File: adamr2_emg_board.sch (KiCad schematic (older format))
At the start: 5 parts, among them J1 Screw_Terminal_01x02, J2 Conn_01x02, J3 Screw_Terminal_01x02, K1 G6C-1114P-US

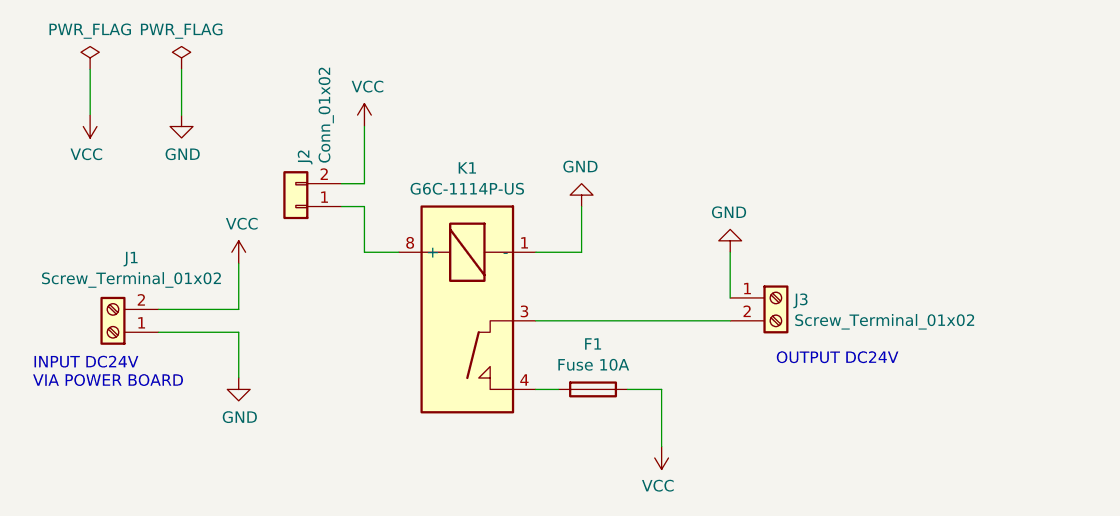
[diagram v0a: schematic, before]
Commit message: Update
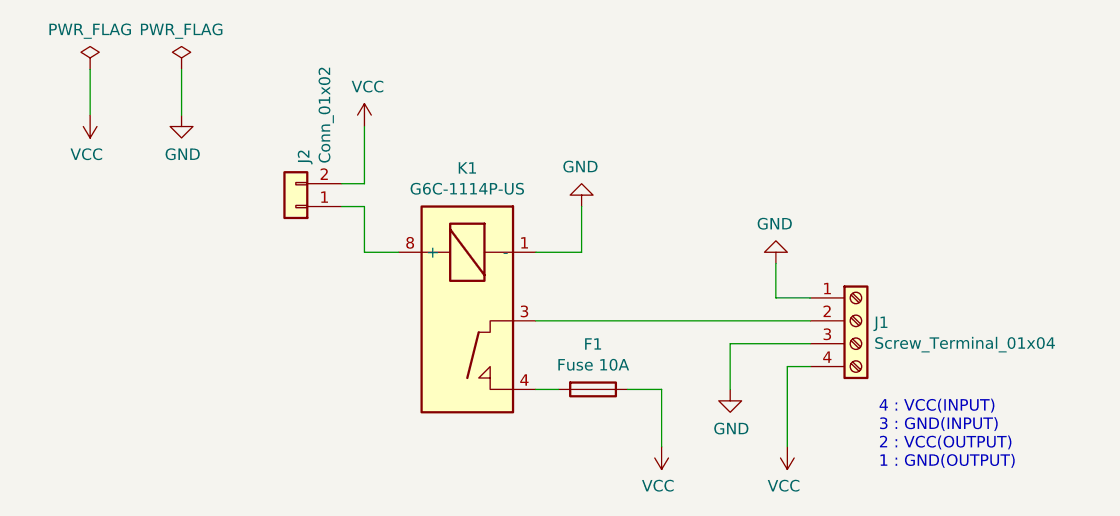
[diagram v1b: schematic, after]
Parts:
- removed J1, J3: Screw_Terminal_01x02, adamr2_footprints:OSTYK21102030, symbol Connector:Screw_Terminal_01x02
- added J1: Screw_Terminal_01x04, adamr2_footprints:OSTYK21104030, symbol Connector:Screw_Terminal_01x04
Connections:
- net GND: now also J1.1 (Pin_1), J1.3 (Pin_3)
- net VCC: now also J1.4 (Pin_4)
- net at K1.3: now also J1.2 (Pin_2)
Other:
- note added: "4 : VCC(INPUT)\n3 : GND(INPUT)\n2 : VCC(OUTPUT)\n1 : GND(OUTPUT)"
- note removed: "INPUT DC24V\nVIA POWER BOARD"
- note removed: "OUTPUT DC24V"
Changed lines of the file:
@@
 L power:GND #PWR02
 U 1 1 5F249FAF
-P 5100 3600
-F 0 "#PWR02" H 5100 3350 50  0001 C CNN
-F 1 "GND" H 5105 3427 50  0000 C CNN
-F 2 "" H 5100 3600 50  0001 C CNN
-F 3 "" H 5100 3600 50  0001 C CNN
-	1    5100 3600
+P 7250 3650
+F 0 "#PWR02" H 7250 3400 50  0001 C CNN
+F 1 "GND" H 7255 3477 50  0000 C CNN
+F 2 "" H 7250 3650 50  0001 C CNN
+F 3 "" H 7250 3650 50  0001 C CNN
+	1    7250 3650
 	1    0    0    -1
 $EndComp
-$Comp
-L Connector:Screw_Terminal_01x02 J1
-U 1 1 5F24A5AD
-P 4550 3400
-F 0 "J1" H 4468 3075 50  0000 C CNN
-F 1 "Screw_Terminal_01x02" H 4468 3166 50  0000 C CNN
-F 2 "adamr2_footprints:OSTYK21102030" H 4550 3400 50  0001 C CNN
-F 3 "~" H 4550 3400 50  0001 C CNN
-	1    4550 3400
-	-1   0    0    1
-$EndComp
-Text Notes 4200 3650 0    50   ~ 0
-INPUT DC24V\nVIA POWER BOARD
 $Comp
 L power:VCC #PWR03
@@
 	-1   0    0    1
 $EndComp
-Text Notes 7450 3550 0    50   ~ 0
-OUTPUT DC24V
 $Comp
 L power:VCC #PWR0102
 U 1 1 5F266BB5
-P 5100 3100
-F 0 "#PWR0102" H 5100 2950 50  0001 C CNN
-F 1 "VCC" H 5115 3273 50  0000 C CNN
-F 2 "" H 5100 3100 50  0001 C CNN
-F 3 "" H 5100 3100 50  0001 C CNN
-	1    5100 3100
-	1    0    0    -1
+P 7500 3900
+F 0 "#PWR0102" H 7500 3750 50  0001 C CNN
+F 1 "VCC" H 7515 4073 50  0000 C CNN
+F 2 "" H 7500 3900 50  0001 C CNN
+F 3 "" H 7500 3900 50  0001 C CNN
+	1    7500 3900
+	-1   0    0    1
 $EndComp
 $Comp
@@
 	4850 2250 4850 2450
 $Comp
-L adamr2_symbols:G6C-1114P-US K1
-U 1 1 5F23BF02
-P 6100 3250
-F 0 "K1" V 5533 3250 50  0000 C CNN
-F 1 "G6C-1114P-US" V 5624 3250 50  0000 C CNN
-F 2 "adamr2_footprints:G6C-1114P-US" H 6450 3200 50  0001 L CNN
-F 3 "https://omronfs.omron.com/ja_JP/ecb/products/pdf/g6c.pdf" H 6100 3250 50  0001 C CNN
-	1    6100 3250
-	0    1    1    0
-$EndComp
-$Comp
 L Connector_Generic:Conn_01x02 J2
 U 1 1 5F24B365
@@
 	5650 2750 5650 2500
 Wire Wire Line
-	4750 3300 5100 3300
-Wire Wire Line
-	5100 3300 5100 3100
-Wire Wire Line
-	5100 3400 5100 3600
-Wire Wire Line
-	4750 3400 5100 3400
-Wire Wire Line
 	6500 3650 6400 3650
-Wire Wire Line
-	7250 3350 6400 3350
 $Comp
 L power:GND #PWR05
 U 1 1 5F254AEA
-P 7250 3050
-F 0 "#PWR05" H 7250 2800 50  0001 C CNN
-F 1 "GND" H 7255 2877 50  0000 C CNN
-F 2 "" H 7250 3050 50  0001 C CNN
-F 3 "" H 7250 3050 50  0001 C CNN
-	1    7250 3050
+P 7450 3100
+F 0 "#PWR05" H 7450 2850 50  0001 C CNN
+F 1 "GND" H 7455 2927 50  0000 C CNN
+F 2 "" H 7450 3100 50  0001 C CNN
+F 3 "" H 7450 3100 50  0001 C CNN
+	1    7450 3100
 	-1   0    0    1
 $EndComp
-$Comp
-L Connector:Screw_Terminal_01x02 J3
-U 1 1 5F24ACF4
-P 7450 3250
-F 0 "J3" H 7530 3242 50  0000 L CNN
-F 1 "Screw_Terminal_01x02" H 7530 3151 50  0000 L CNN
-F 2 "adamr2_footprints:OSTYK21102030" H 7450 3250 50  0001 C CNN
-F 3 "~" H 7450 3250 50  0001 C CNN
-	1    7450 3250
-	1    0    0    -1
-$EndComp
-Wire Wire Line
-	7250 3050 7250 3250
 Wire Wire Line
 	6800 3650 6950 3650
 Wire Wire Line
 	6950 3650 6950 3900
+$Comp
+L Connector:Screw_Terminal_01x04 J1
+U 1 1 5F2A9452
+P 7800 3350
+F 0 "J1" H 7880 3342 50  0000 L CNN
+F 1 "Screw_Terminal_01x04" H 7880 3251 50  0000 L CNN
+F 2 "adamr2_footprints:OSTYK21104030" H 7800 3350 50  0001 C CNN
+F 3 "~" H 7800 3350 50  0001 C CNN
+	1    7800 3350
+	1    0    0    -1
+$EndComp
+Text Notes 7900 4000 0    50   ~ 0
+4 : VCC(INPUT)\n3 : GND(INPUT)\n2 : VCC(OUTPUT)\n1 : GND(OUTPUT)
+Wire Wire Line
+	6400 3350 7600 3350
+Wire Wire Line
+	7450 3100 7450 3250
+Wire Wire Line
+	7450 3250 7600 3250
+Wire Wire Line
+	7600 3550 7500 3550
+Wire Wire Line
+	7500 3550 7500 3900
+Wire Wire Line
+	7600 3450 7250 3450
+Wire Wire Line
+	7250 3450 7250 3650
+$Comp
+L adamr2_symbols:G6C-1114P-US K1
+U 1 1 5F23BF02
+P 6100 3250
+F 0 "K1" V 5533 3250 50  0000 C CNN
+F 1 "G6C-1114P-US" V 5624 3250 50  0000 C CNN
+F 2 "adamr2_footprints:G6C-1114P-US" H 6450 3200 50  0001 L CNN
+F 3 "https://omronfs.omron.com/ja_JP/ecb/products/pdf/g6c.pdf" H 6100 3250 50  0001 C CNN
+	1    6100 3250
+	0    1    1    0
+$EndComp
 $EndSCHEMATC

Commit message: Update: ヒューズホルダの種類を変更した
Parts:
- F1: footprint adamr2_footprints:FUC-03A -> adamr2_footprints:F-60-A
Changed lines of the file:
@@
 F 0 "F1" V 6453 3650 50  0000 C CNN
 F 1 "Fuse 10A" V 6544 3650 50  0000 C CNN
-F 2 "adamr2_footprints:FUC-03A" V 6580 3650 50  0001 C CNN
+F 2 "adamr2_footprints:F-60-A" V 6580 3650 50  0001 C CNN
 F 3 "~" H 6650 3650 50  0001 C CNN
 	1    6650 3650
